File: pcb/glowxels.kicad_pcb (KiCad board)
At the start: 2 copper layers, 79 parts, among them J1 OUT, J2 IN, U1 STP16CPC26, U2 STP16CPC26, U3 STP16CPC26, U4 STP16CPC26

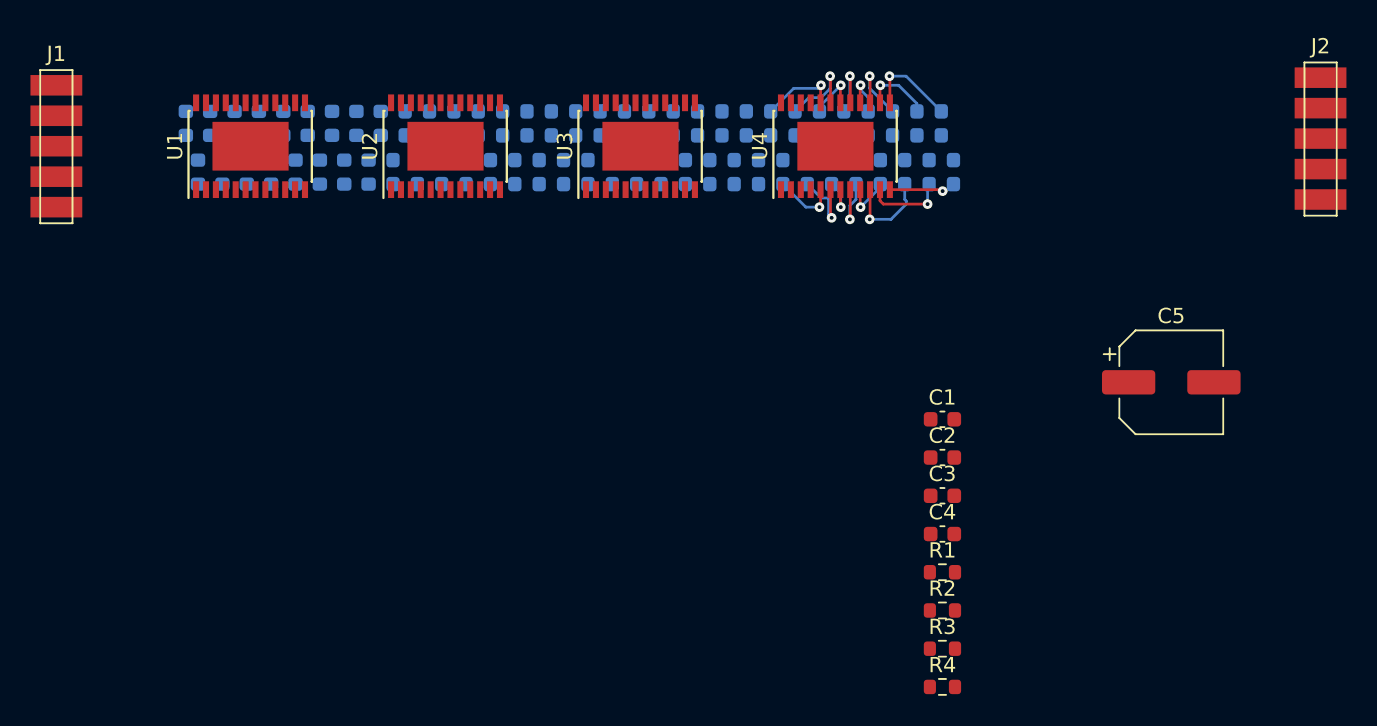
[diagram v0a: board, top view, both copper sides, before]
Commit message: First version, fully routed.
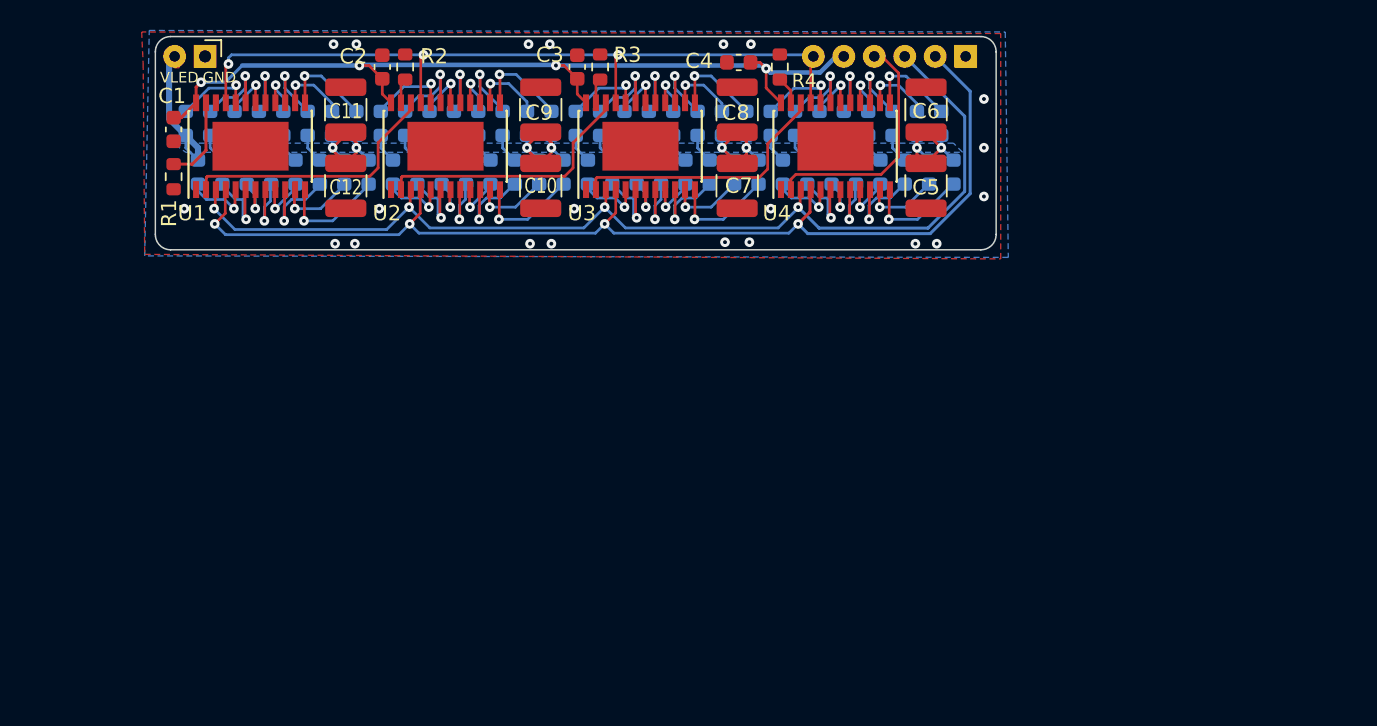
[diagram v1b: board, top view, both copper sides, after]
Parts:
- added C10: 47u, Capacitor_SMD:C_1210_3225Metric, F.Cu at (73.3, 49.1)
- added C11: 47u, Capacitor_SMD:C_1210_3225Metric, F.Cu at (60.5, 44.1)
- added C12: 47u, Capacitor_SMD:C_1210_3225Metric, F.Cu at (60.5, 49.1)
- added C6: 47u, Capacitor_SMD:C_1210_3225Metric, F.Cu at (98.6, 44.1)
- added C7: 47u, Capacitor_SMD:C_1210_3225Metric, F.Cu at (86.2, 49.1)
- added C8: 47u, Capacitor_SMD:C_1210_3225Metric, F.Cu at (86.2, 44.1)
- added C9: 47u, Capacitor_SMD:C_1210_3225Metric, F.Cu at (73.3, 44.1)
- C5: value 100u -> 47u; footprint Capacitor_SMD:CP_Elec_6.3x5.3 -> Capacitor_SMD:C_1210_3225Metric
- J1: value OUT -> Conn_01x06_Pin; footprint Glowxels:EdgeConnect -> Connector_PinHeader_2.00mm:PinHeader_1x06_P2.00mm_Vertical
- J2: value IN -> Conn_01x02_Pin; footprint Glowxels:EdgeConnect -> Connector_PinHeader_2.00mm:PinHeader_1x02_P2.00mm_Vertical
- moved J2 73.2 mm to (51.3, 40.6), turned to -90 degrees
- moved J1 59.7 mm to (101.2, 40.6), turned to -90 degrees
- moved R1 56.8 mm to (49.2, 48.5), turned to 90 degrees
- moved C1 53.9 mm to (49.2, 45.4), turned to -90 degrees
- moved R2 50.2 mm to (64.4, 41.3), turned to -90 degrees
- moved C2 44.8 mm to (62.9, 41.3), turned to 90 degrees
- moved R3 44.3 mm to (77.2, 41.3), turned to -90 degrees
- moved R4 42.1 mm to (89.0, 41.3), turned to -90 degrees
- moved C3 37.0 mm to (75.7, 41.3), turned to 90 degrees
- moved C4 33.7 mm to (86.3, 41.0), turned to 180 degrees
- moved C5 20.6 mm to (98.6, 49.1), turned to -90 degrees
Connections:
- J1 pad 1: /VDD -> GND
- J1 pad 2: /D-Out -> /Latch
- J1 pad 3: /~{OE} -> /CLK
- J1 pad 4: /CLK -> /D-IN
- J1 pad 5: /Latch -> /VDD
- J2 pad 1: /VDD -> GND
- J2 pad 2: /D-IN -> /LED-Power
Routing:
- net /LED-Power: track 0.00 -> 92.4 mm, vias 0 -> 8
- net /Latch: track 0.00 -> 72.7 mm, vias 0 -> 4
- net /CLK: track 0.00 -> 69.6 mm, vias 0 -> 4
- net /VDD: track 0.00 -> 58.1 mm, vias 0 -> 4
- net /~{OE}: track 0.00 -> 52.9 mm, vias 0 -> 3
- net Net-(U3-SDI): track 0.00 -> 17.5 mm
- net Net-(U1-SDI): track 0.00 -> 17.5 mm
- net Net-(U2-SDI): track 0.00 -> 17.5 mm
- net /D-IN: track 0.00 -> 15.9 mm
- net Net-(D9-K): track 0.00 -> 7.12 mm, vias 0 -> 1
- net Net-(D41-K): track 0.00 -> 7.12 mm, vias 0 -> 1
- net Net-(D25-K): track 0.00 -> 7.12 mm, vias 0 -> 1
- net Net-(D8-K): track 0.00 -> 6.12 mm, vias 0 -> 1
- net Net-(D24-K): track 0.00 -> 6.12 mm, vias 0 -> 1
- net Net-(D40-K): track 0.00 -> 6.12 mm, vias 0 -> 1
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- added copper zone on B.Cu, net /LED-Power
- added copper zone on B.Cu, net GND
- added copper zone on F.Cu, net GND
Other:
- board outline added: 55.2 x 14 mm
- board text added: "CLK"
- board text added: "DIN"
- board text added: "GND"
- board text added: "LAT"
- board text added: "VCC"
- board text added: "VLED"
- board text added: "~{OE}"
